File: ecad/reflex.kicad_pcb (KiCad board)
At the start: 2 copper layers, 20 x 55 mm, 26 parts, among them J1 USB_MICRO_B_SMD_2, J2 CONN_02X04_RA, Q1 BPW85C, SW1 CHERRY_MX1A-E1NW_BLUE, SW2 B3U-3000P_SPST-NO_SMD, U1 USBLC6, U2 ATSAMD21E18A, U3 AP2112K-3.3, U4 APA102-2020, U5 APA102-2020, X1 SWD_SMT_SOCKET

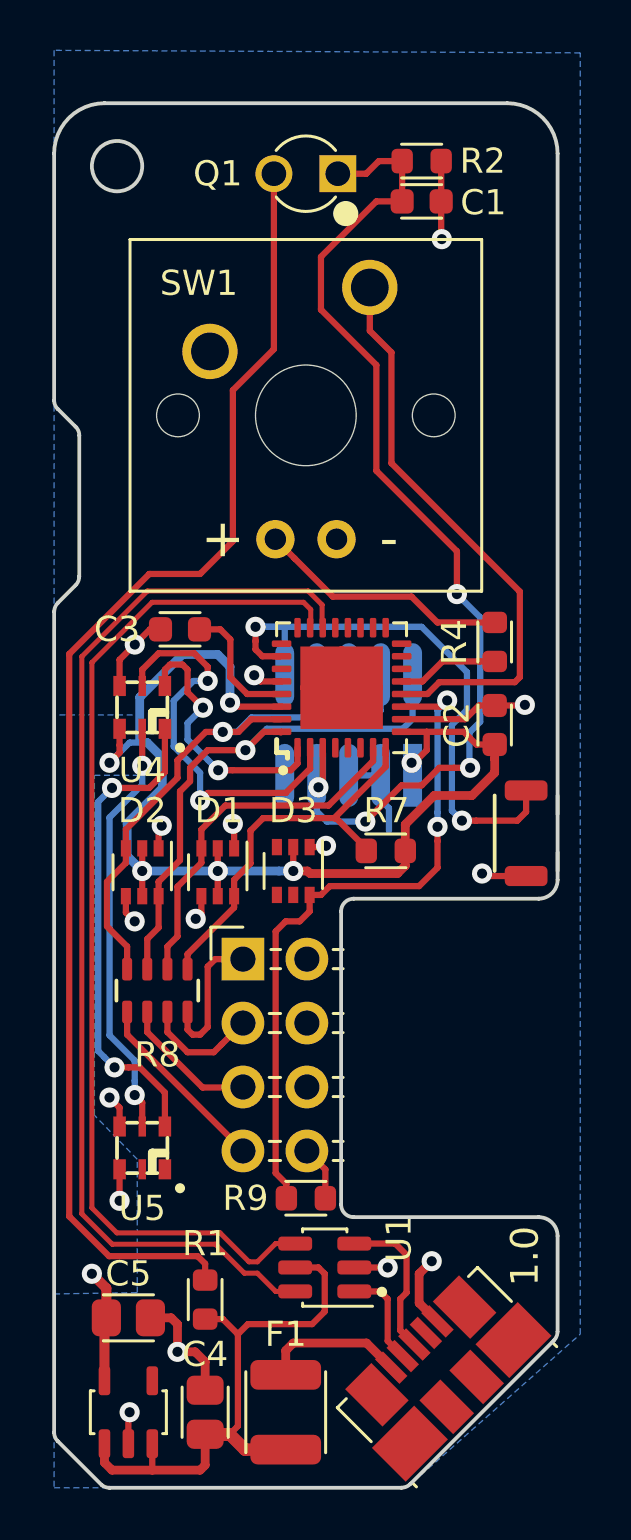
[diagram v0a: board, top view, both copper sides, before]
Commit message: Adds gerber exports
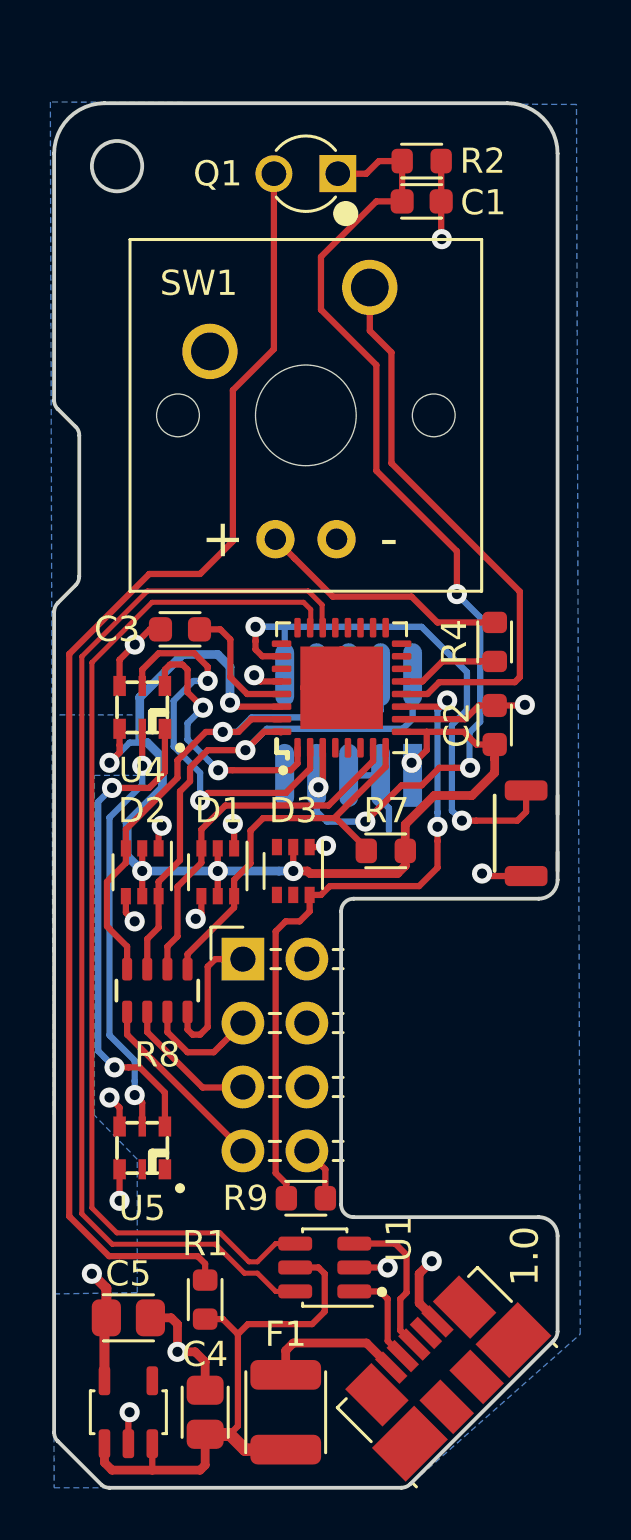
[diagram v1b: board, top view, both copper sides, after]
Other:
- board text added: "Board Stackup 55x20 mm 1.6mm or 2.0mm thick FR4 2 layer, 35um (1 oz) copper ENIG or HASL finish OK Green soldermask White silkscreen"
- board text removed: "Board Stackup 55x20 mm 1.6mm or 2.0mm thick FR4 2 layer, 35um (1 oz) copper ENIG or HASL finish OK"
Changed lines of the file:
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@@
     (visible_elements FFFFFF7F)
     (pcbplotparams
-      (layerselection 0x010fc_ffffffff)
-      (usegerberextensions false)
+      (layerselection 0x213f0_ffffffff)
+      (usegerberextensions true)
       (usegerberattributes false)
       (usegerberadvancedattributes false)
@@
       (outputformat 1)
       (mirror false)
-      (drillshape 1)
+      (drillshape 0)
       (scaleselection 1)
-      (outputdirectory ""))
+      (outputdirectory "outputs/"))
   )
   (net 0 "")
@@
     )
   )
-  (gr_text "Board Stackup\n\n55x20 mm\n1.6mm or 2.0mm thick FR4\n2 layer, 35um (1 oz) copper\nENIG or HASL finish OK\n" (at 135.8 96) (layer Cmts.User)
+  (gr_text "Board Stackup\n\n55x20 mm\n1.6mm or 2.0mm thick FR4\n2 layer, 35um (1 oz) copper\nENIG or HASL finish OK\n\nGreen soldermask\nWhite silkscreen" (at 135.8 96) (layer Cmts.User)
     (effects (font (size 3 3) (thickness 0.3)) (justify left))
   )
@@
     (polygon
       (pts
-        (xy 90 130) (xy 104 130) (xy 110.9 123.9) (xy 110.9 73) (xy 90 72.9)
+        (xy 90 130) (xy 104 130) (xy 110.9 123.9) (xy 110.75 75.05) (xy 89.85 74.95)
       )
     )
